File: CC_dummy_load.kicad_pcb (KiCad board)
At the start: 2 copper layers, 109.9 x 99.6 mm, 67 parts, among them P1 CONN_01X02, P2 12vFAN, P3 Arduino_Nano, P4 LOAD, P5 KeyPad, P6 LCD_I2C, Q1 Darl_NPN, Q2 IRF540N, U1 LM324N, U2 MCP4921-E/P, U3 LM35

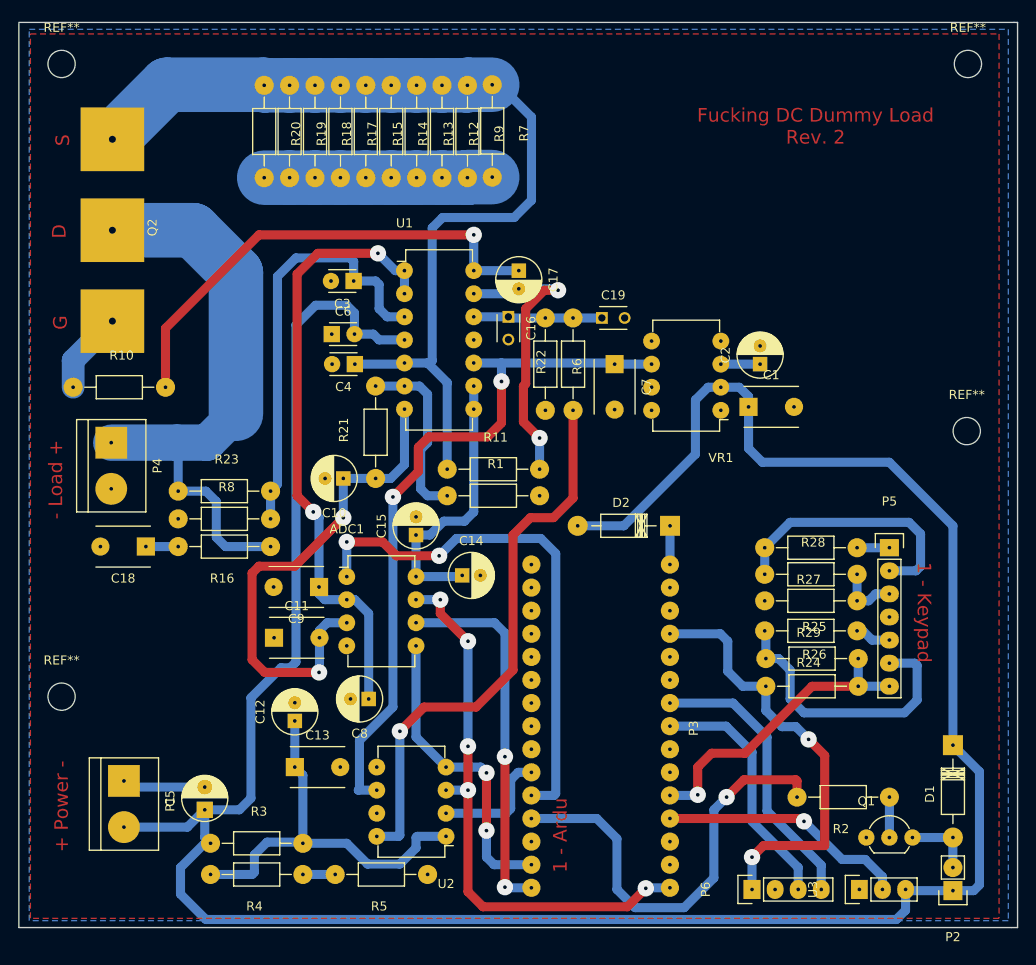
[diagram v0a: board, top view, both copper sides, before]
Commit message: Revert "mounting holes and stuff"
This reverts commit a6e826f9ddd28fcc19281836c77182ce96cc9986.
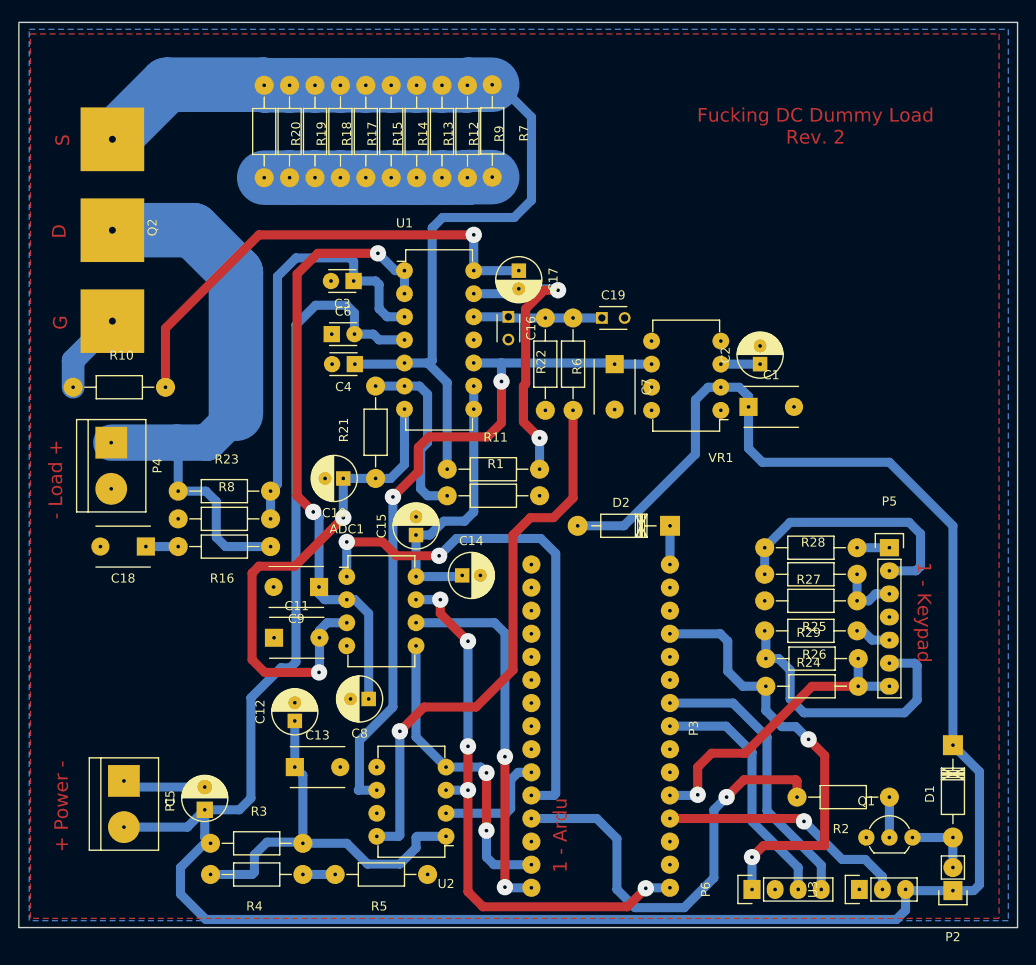
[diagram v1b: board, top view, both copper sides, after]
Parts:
- removed REF** (x4): MountingHole_3mm, Mounting_Holes:MountingHole_3mm
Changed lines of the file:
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@@
     (links 136)
     (no_connects 1)
-    (area 36.210474 30.9695 151.084046 133.302)
+    (area 37.897999 31.420999 198.068001 133.302)
     (thickness 1.6)
     (drawings 14)
     (tracks 379)
     (zones 0)
-    (modules 67)
+    (modules 63)
     (nets 59)
   )
@@
   )
   (setup
-    (last_trace_width 0.6)
+    (last_trace_width 1)
     (user_trace_width 0.6)
     (user_trace_width 0.8)
@@
     (visible_elements FFFFFF7F)
     (pcbplotparams
-      (layerselection 0x00000_7fffffff)
+      (layerselection 0x00000_fffffffe)
       (usegerberextensions false)
       (excludeedgelayer false)
@@
       (drillshape 2)
       (scaleselection 1)
-      (outputdirectory /home/paco/tmp/))
+      (outputdirectory ""))
   )
   (net 0 "")
@@
     )
   )
-  (module Mounting_Holes:MountingHole_3mm (layer F.Cu)
-    (at 142.494 36.195)
-    (descr "Mounting hole, Befestigungsbohrung, 3mm, No Annular, Kein Restring,")
-    (tags "Mounting hole, Befestigungsbohrung, 3mm, No Annular, Kein Restring,")
-    (fp_text reference REF** (at 0 -4.0005) (layer F.SilkS)
-      (effects (font (size 1 1) (thickness 0.15)))
-    )
-    (fp_text value MountingHole_3mm (at 1.00076 5.00126) (layer F.Fab)
-      (effects (font (size 1 1) (thickness 0.15)))
-    )
-    (fp_circle (center 0 0) (end 3 0) (layer Cmts.User) (width 0.381))
-    (pad 1 thru_hole circle (at 0 0) (size 3 3) (drill 3) (layers))
-  )
-  (module Mounting_Holes:MountingHole_3mm (layer F.Cu)
-    (at 42.799 36.195)
-    (descr "Mounting hole, Befestigungsbohrung, 3mm, No Annular, Kein Restring,")
-    (tags "Mounting hole, Befestigungsbohrung, 3mm, No Annular, Kein Restring,")
-    (fp_text reference REF** (at 0 -4.0005) (layer F.SilkS)
-      (effects (font (size 1 1) (thickness 0.15)))
-    )
-    (fp_text value MountingHole_3mm (at 1.00076 5.00126) (layer F.Fab)
-      (effects (font (size 1 1) (thickness 0.15)))
-    )
-    (fp_circle (center 0 0) (end 3 0) (layer Cmts.User) (width 0.381))
-    (pad 1 thru_hole circle (at 0 0) (size 3 3) (drill 3) (layers))
-  )
-  (module Mounting_Holes:MountingHole_3mm (layer F.Cu)
-    (at 42.799 105.791)
-    (descr "Mounting hole, Befestigungsbohrung, 3mm, No Annular, Kein Restring,")
-    (tags "Mounting hole, Befestigungsbohrung, 3mm, No Annular, Kein Restring,")
-    (fp_text reference REF** (at 0 -4.0005) (layer F.SilkS)
-      (effects (font (size 1 1) (thickness 0.15)))
-    )
-    (fp_text value MountingHole_3mm (at 1.00076 5.00126) (layer F.Fab)
-      (effects (font (size 1 1) (thickness 0.15)))
-    )
-    (fp_circle (center 0 0) (end 3 0) (layer Cmts.User) (width 0.381))
-    (pad 1 thru_hole circle (at 0 0) (size 3 3) (drill 3) (layers))
-  )
-  (module Mounting_Holes:MountingHole_3mm (layer F.Cu)
-    (at 142.367 76.581)
-    (descr "Mounting hole, Befestigungsbohrung, 3mm, No Annular, Kein Restring,")
-    (tags "Mounting hole, Befestigungsbohrung, 3mm, No Annular, Kein Restring,")
-    (fp_text reference REF** (at 0 -4.0005) (layer F.SilkS)
-      (effects (font (size 1 1) (thickness 0.15)))
-    )
-    (fp_text value MountingHole_3mm (at 1.00076 5.00126) (layer F.Fab)
-      (effects (font (size 1 1) (thickness 0.15)))
-    )
-    (fp_circle (center 0 0) (end 3 0) (layer Cmts.User) (width 0.381))
-    (pad 1 thru_hole circle (at 0 0) (size 3 3) (drill 3) (layers))
-  )
   (gr_line (start 147.955 131.191) (end 147.32 131.191) (angle 90) (layer Edge.Cuts) (width 0.15))

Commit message: mounting holes and stuff
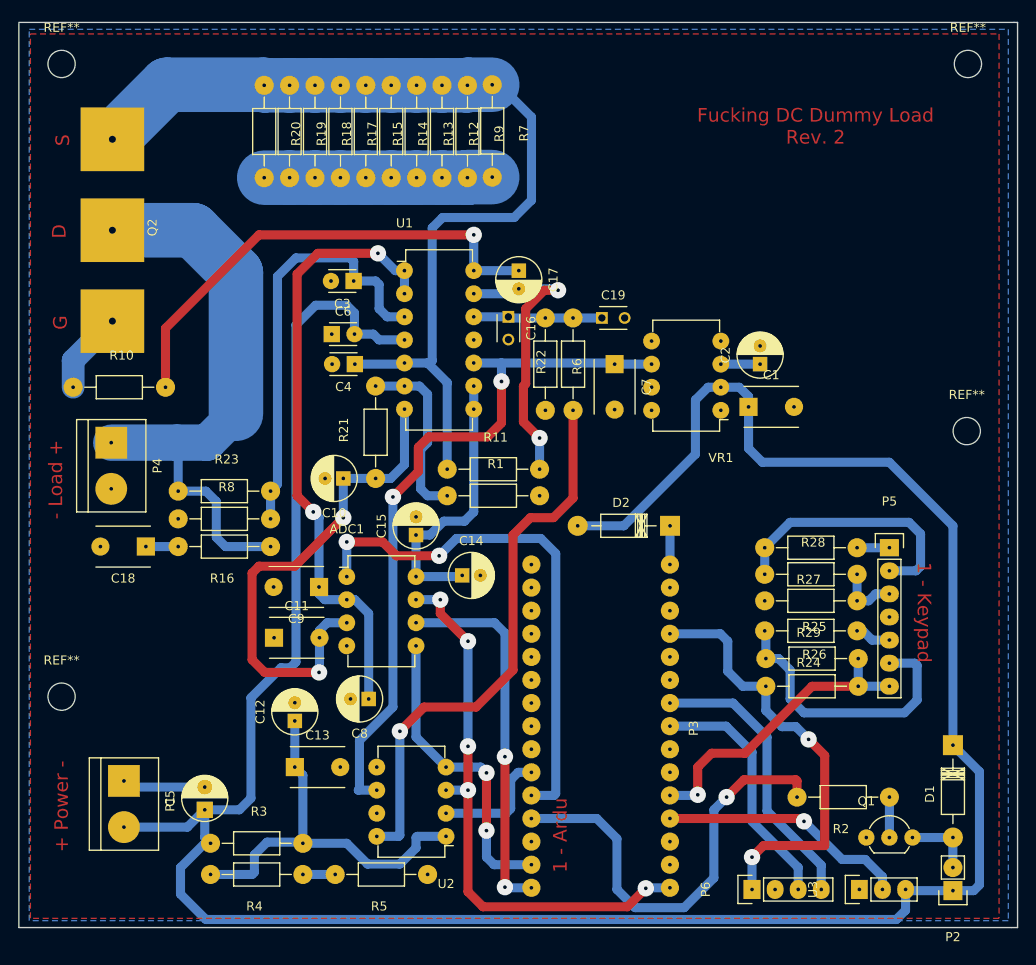
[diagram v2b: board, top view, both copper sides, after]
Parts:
- added REF**: MountingHole_3mm, Mounting_Holes:MountingHole_3mm, F.Cu at (142.5, 36.2)
- added REF**: MountingHole_3mm, Mounting_Holes:MountingHole_3mm, F.Cu at (42.8, 36.2)
- added REF**: MountingHole_3mm, Mounting_Holes:MountingHole_3mm, F.Cu at (42.8, 105.8)
- added REF**: MountingHole_3mm, Mounting_Holes:MountingHole_3mm, F.Cu at (142.4, 76.6)
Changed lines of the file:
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@@
     (links 136)
     (no_connects 1)
-    (area 37.897999 31.420999 198.068001 133.302)
+    (area 36.210474 30.9695 151.084046 133.302)
     (thickness 1.6)
     (drawings 14)
     (tracks 379)
     (zones 0)
-    (modules 63)
+    (modules 67)
     (nets 59)
   )
@@
   )
   (setup
-    (last_trace_width 1)
+    (last_trace_width 0.6)
     (user_trace_width 0.6)
     (user_trace_width 0.8)
@@
     (visible_elements FFFFFF7F)
     (pcbplotparams
-      (layerselection 0x00000_fffffffe)
+      (layerselection 0x00000_7fffffff)
       (usegerberextensions false)
       (excludeedgelayer false)
@@
       (drillshape 2)
       (scaleselection 1)
-      (outputdirectory ""))
+      (outputdirectory /home/paco/tmp/))
   )
   (net 0 "")
@@
     )
   )
+  (module Mounting_Holes:MountingHole_3mm (layer F.Cu)
+    (at 142.494 36.195)
+    (descr "Mounting hole, Befestigungsbohrung, 3mm, No Annular, Kein Restring,")
+    (tags "Mounting hole, Befestigungsbohrung, 3mm, No Annular, Kein Restring,")
+    (fp_text reference REF** (at 0 -4.0005) (layer F.SilkS)
+      (effects (font (size 1 1) (thickness 0.15)))
+    )
+    (fp_text value MountingHole_3mm (at 1.00076 5.00126) (layer F.Fab)
+      (effects (font (size 1 1) (thickness 0.15)))
+    )
+    (fp_circle (center 0 0) (end 3 0) (layer Cmts.User) (width 0.381))
+    (pad 1 thru_hole circle (at 0 0) (size 3 3) (drill 3) (layers))
+  )
+  (module Mounting_Holes:MountingHole_3mm (layer F.Cu)
+    (at 42.799 36.195)
+    (descr "Mounting hole, Befestigungsbohrung, 3mm, No Annular, Kein Restring,")
+    (tags "Mounting hole, Befestigungsbohrung, 3mm, No Annular, Kein Restring,")
+    (fp_text reference REF** (at 0 -4.0005) (layer F.SilkS)
+      (effects (font (size 1 1) (thickness 0.15)))
+    )
+    (fp_text value MountingHole_3mm (at 1.00076 5.00126) (layer F.Fab)
+      (effects (font (size 1 1) (thickness 0.15)))
+    )
+    (fp_circle (center 0 0) (end 3 0) (layer Cmts.User) (width 0.381))
+    (pad 1 thru_hole circle (at 0 0) (size 3 3) (drill 3) (layers))
+  )
+  (module Mounting_Holes:MountingHole_3mm (layer F.Cu)
+    (at 42.799 105.791)
+    (descr "Mounting hole, Befestigungsbohrung, 3mm, No Annular, Kein Restring,")
+    (tags "Mounting hole, Befestigungsbohrung, 3mm, No Annular, Kein Restring,")
+    (fp_text reference REF** (at 0 -4.0005) (layer F.SilkS)
+      (effects (font (size 1 1) (thickness 0.15)))
+    )
+    (fp_text value MountingHole_3mm (at 1.00076 5.00126) (layer F.Fab)
+      (effects (font (size 1 1) (thickness 0.15)))
+    )
+    (fp_circle (center 0 0) (end 3 0) (layer Cmts.User) (width 0.381))
+    (pad 1 thru_hole circle (at 0 0) (size 3 3) (drill 3) (layers))
+  )
+  (module Mounting_Holes:MountingHole_3mm (layer F.Cu)
+    (at 142.367 76.581)
+    (descr "Mounting hole, Befestigungsbohrung, 3mm, No Annular, Kein Restring,")
+    (tags "Mounting hole, Befestigungsbohrung, 3mm, No Annular, Kein Restring,")
+    (fp_text reference REF** (at 0 -4.0005) (layer F.SilkS)
+      (effects (font (size 1 1) (thickness 0.15)))
+    )
+    (fp_text value MountingHole_3mm (at 1.00076 5.00126) (layer F.Fab)
+      (effects (font (size 1 1) (thickness 0.15)))
+    )
+    (fp_circle (center 0 0) (end 3 0) (layer Cmts.User) (width 0.381))
+    (pad 1 thru_hole circle (at 0 0) (size 3 3) (drill 3) (layers))
+  )
   (gr_line (start 147.955 131.191) (end 147.32 131.191) (angle 90) (layer Edge.Cuts) (width 0.15))
